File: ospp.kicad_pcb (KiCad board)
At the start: 2 copper layers, 63.5 x 71.1 mm, 43 parts, among them U1 L7815, U2 OpAmp

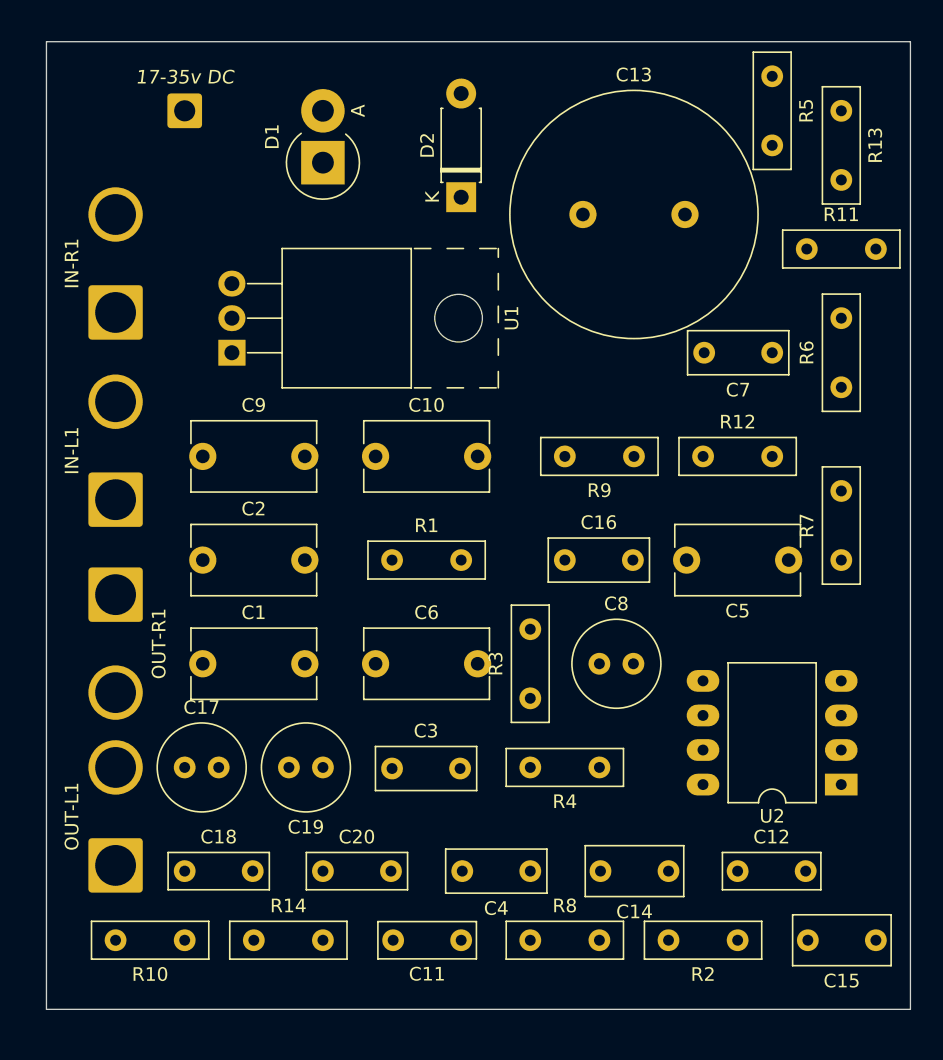
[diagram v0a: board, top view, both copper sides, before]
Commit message: Add files via upload
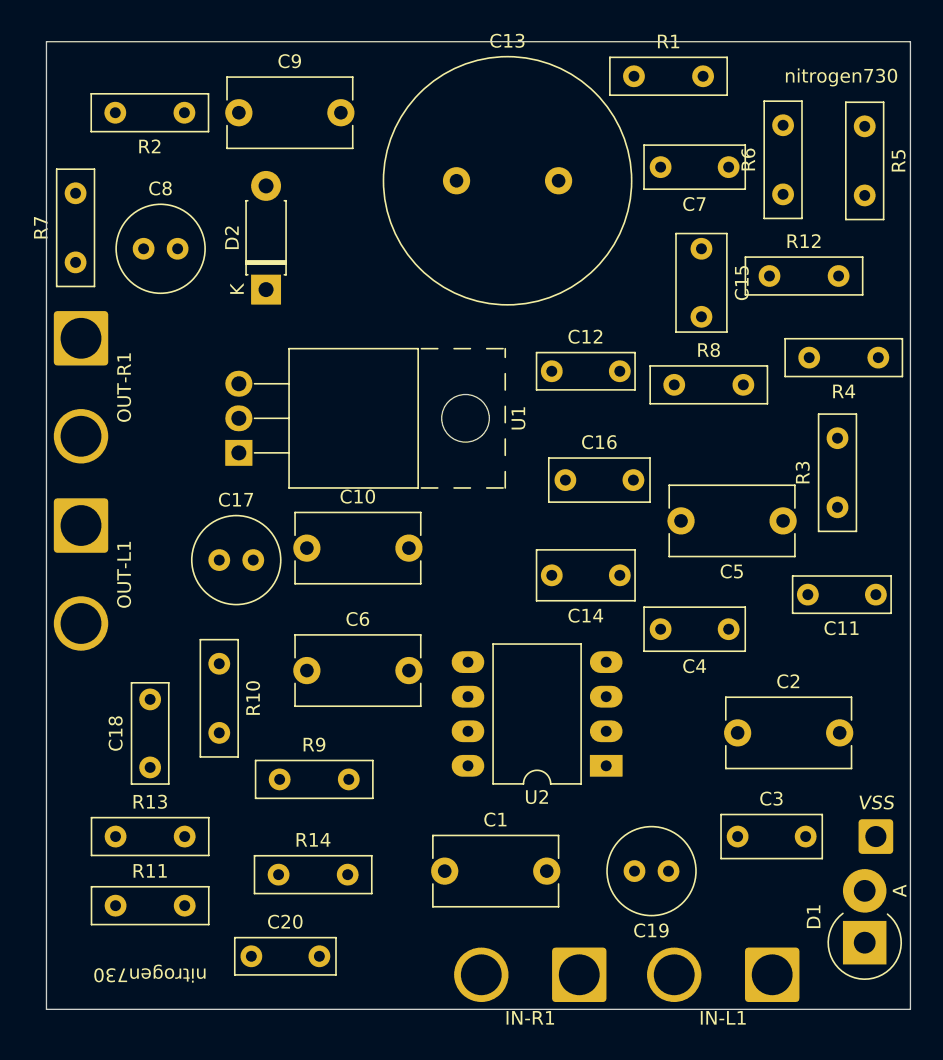
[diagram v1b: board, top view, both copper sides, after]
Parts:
- VSS: renamed from 17-35v DC
- moved R13 75.4 mm to (27.9, 76.2), turned to 0 degrees
- moved VSS 73.7 mm to (83.8, 76.2)
- moved R2 73.2 mm to (33.0, 23.0)
- moved R11 70.1 mm to (27.9, 81.3)
- moved D1 69.8 mm to (83.0, 84.0)
- moved R7 60.4 mm to (25.0, 34.0)
- moved IN-L1 59.6 mm to (76.2, 86.4), turned to 180 degrees
- moved IN-R1 59.4 mm to (62.0, 86.4), turned to 180 degrees
- moved C15 52.4 mm to (71.0, 33.0), turned to -90 degrees
- moved C8 45.3 mm to (30.0, 33.0)
- moved R8 42.2 mm to (69.0, 43.0)
- moved C2 41.3 mm to (73.7, 68.6)
- moved R1 39.8 mm to (66.0, 20.3)
- moved C11 39.7 mm to (83.8, 58.4)
- moved C12 39.2 mm to (60.0, 42.0)
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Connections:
- VSS pad 1: (no net) -> VSS
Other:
- board text added: "nitrogen730"
